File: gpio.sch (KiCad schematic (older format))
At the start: 7 parts, among them J1 DF40C-100DP-0.4V(51), J2 DF40C-100DP-0.4V(51), U1 LFE5U-85F-6BG381C

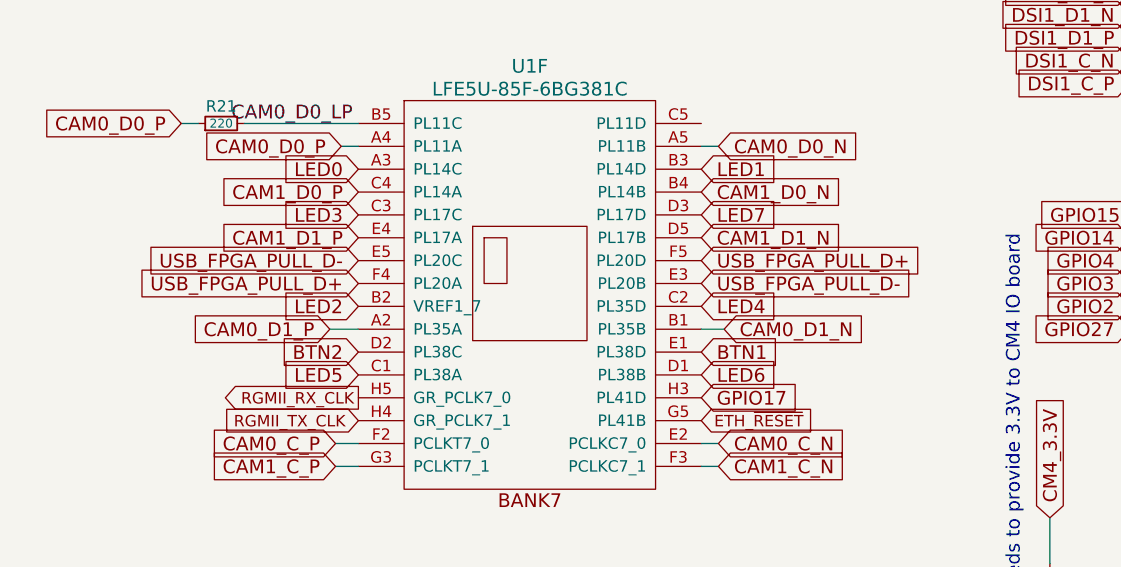
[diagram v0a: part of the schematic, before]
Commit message: Changing and routing USB pins fix #25
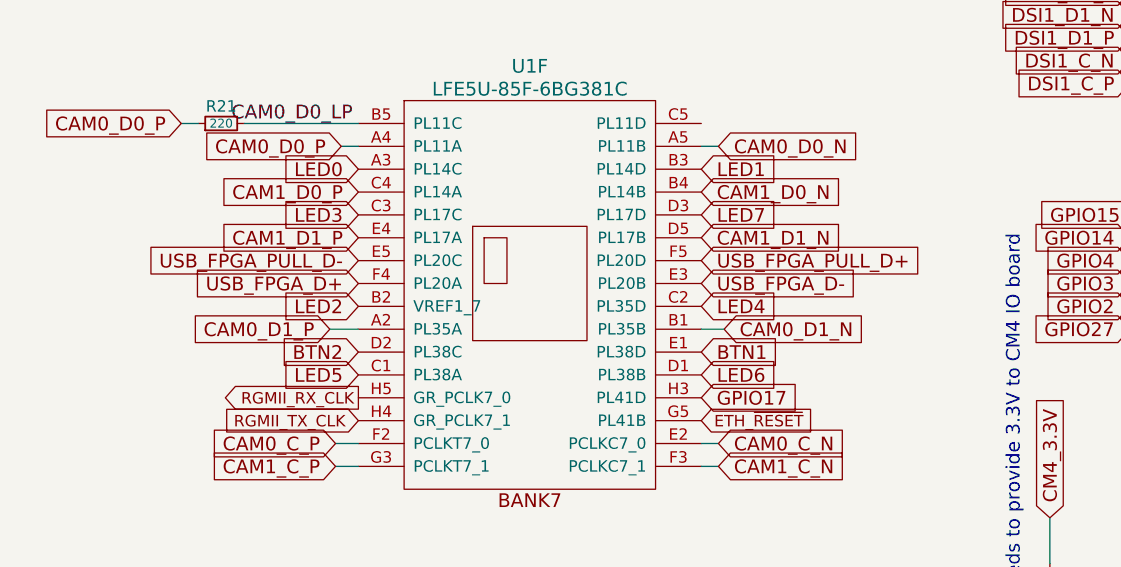
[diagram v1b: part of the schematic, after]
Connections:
- net USB_FPGA_D+: now also U1.F4 (PL20A)
- net USB_FPGA_D-: now also U1.E3 (PL20B)
- net USB_FPGA_PULL_D+: no longer U1.F4 (PL20A)
- net USB_FPGA_PULL_D-: no longer U1.E3 (PL20B)
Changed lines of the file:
@@
 LED1
 Text GLabel 1925 3950 0    60   Input ~ 0
-USB_FPGA_PULL_D+
+USB_FPGA_D+
 Text GLabel 3425 3950 2    60   Input ~ 0
-USB_FPGA_PULL_D-
+USB_FPGA_D-
 Text GLabel 1825 4750 0    60   Input ~ 0
 CAM1_C_P

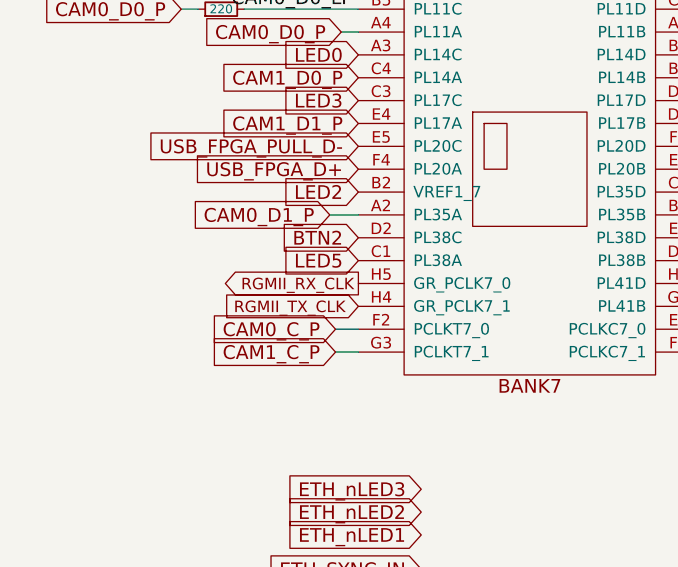
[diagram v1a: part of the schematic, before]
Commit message: Chaning RGMII_RX_CLK to H2, removing H5, adding pulldown to pin 33 fix #35
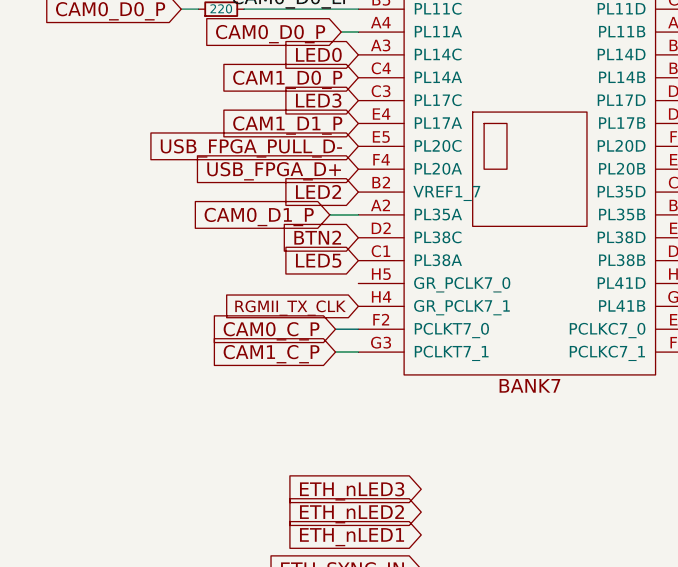
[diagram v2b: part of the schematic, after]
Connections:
- net RGMII_RX_CLK: no longer names the net of U1.H5 (GR_PCLK7_0)
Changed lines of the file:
@@
 Text GLabel 3425 4450 2    60   Input ~ 0
 GPIO17
-Text GLabel 1925 4450 0    50   Output ~ 0
-RGMII_RX_CLK
 Text GLabel 1925 4550 0    50   Input ~ 0
 RGMII_TX_CLK

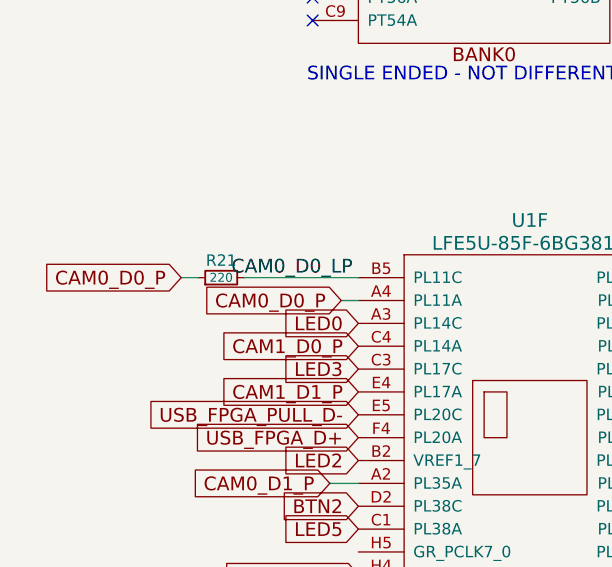
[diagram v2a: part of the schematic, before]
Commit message: Lowering number of unique parts fix #37
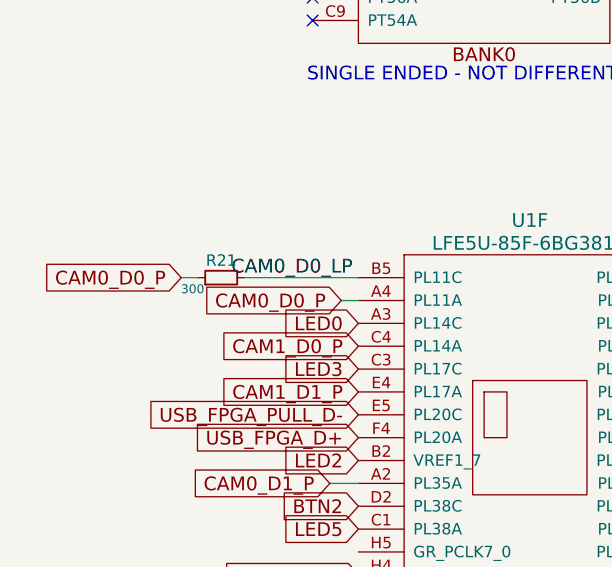
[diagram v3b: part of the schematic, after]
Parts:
- R21: value 220 -> 300
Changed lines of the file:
@@
 AR Path="/56AC389C/625E5FDB" Ref="R21"  Part="1"
 F 0 "R21" V 1400 3250 50  0000 C CNN
-F 1 "220" V 1325 3250 39  0000 C CNN
+F 1 "300" V 1275 3375 39  0000 C CNN
 F 2 "Resistor_SMD:R_0402_1005Metric" H 1325 3250 50  0001 C CNN
 F 3 "~" H 1325 3250 50  0001 C CNN

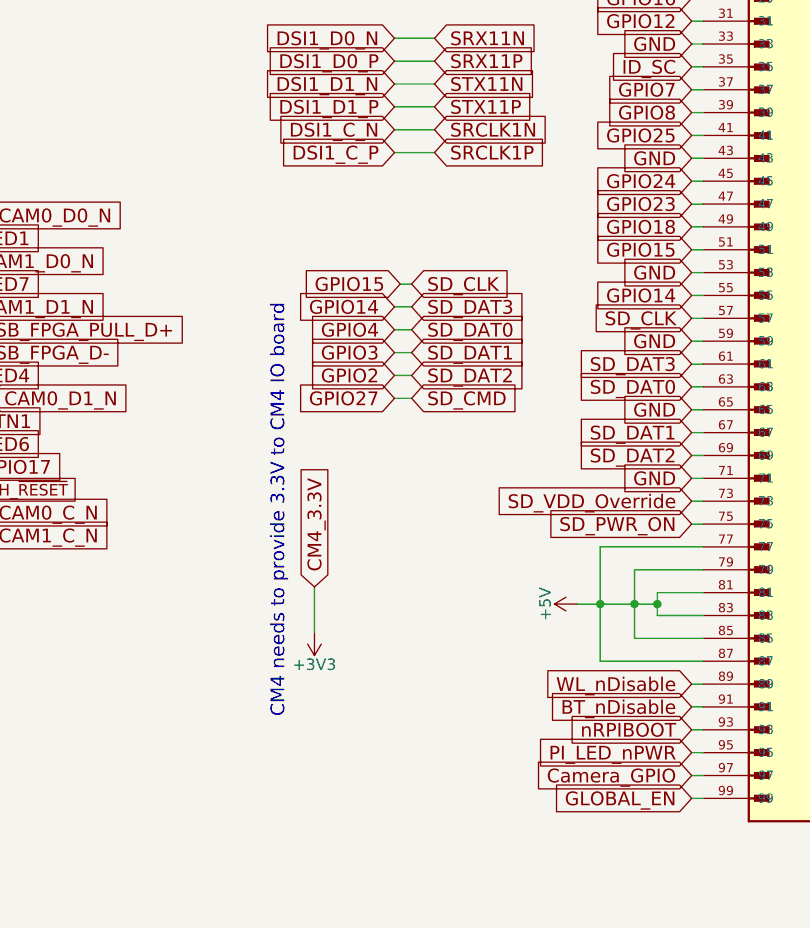
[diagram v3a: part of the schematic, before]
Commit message: Removing SD-CARD sharing feature to get more GPIO pins
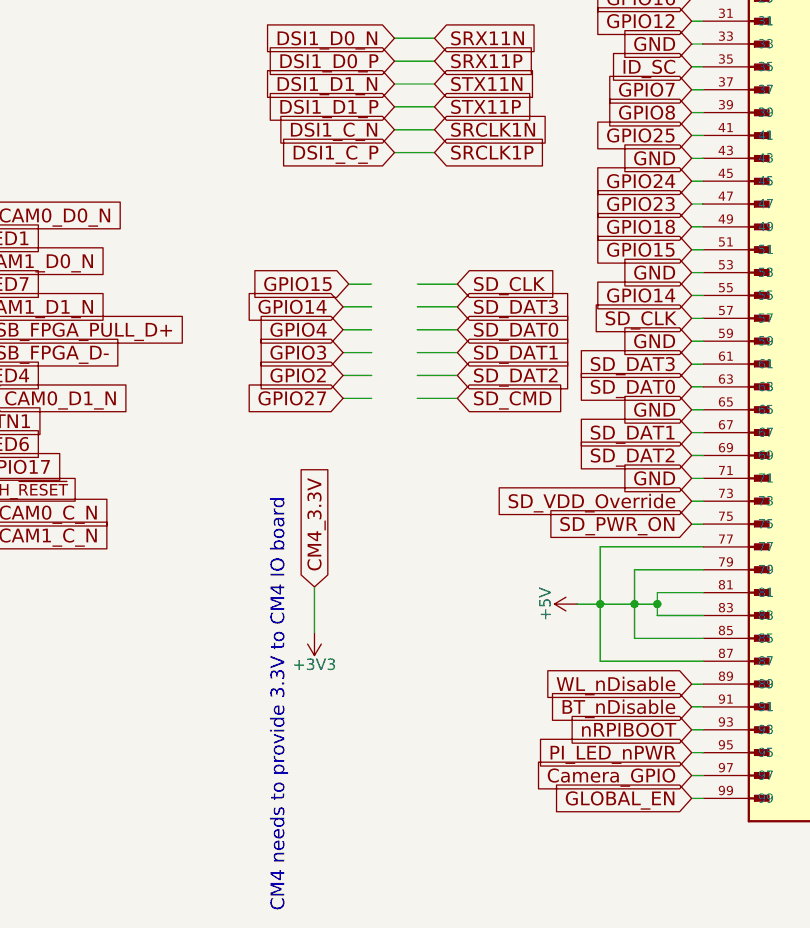
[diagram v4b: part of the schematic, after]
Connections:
- wire segments 232 -> 238
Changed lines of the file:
@@
 Wire Wire Line
 	4950 5175 4950 4975
-Text Notes 4825 5550 1    60   ~ 0
+Text Notes 4825 6400 1    60   ~ 0
 CM4 needs to provide 3.3V to CM4 IO board
 Text GLabel 5475 2675 2    60   Input ~ 0
@@
 Wire Wire Line
 	5475 3075 5300 3075
-Text GLabel 5325 3650 0    60   Input ~ 0
+Text GLabel 5100 3650 0    60   Input ~ 0
 GPIO15
-Text GLabel 5375 3650 2    60   Input ~ 0
+Text GLabel 5575 3650 2    60   Input ~ 0
 SD_CLK
-Wire Wire Line
-	5325 3650 5375 3650
-Text GLabel 5300 3750 0    60   Input ~ 0
+Text GLabel 5075 3750 0    60   Input ~ 0
 GPIO14
-Text GLabel 5375 3750 2    60   Input ~ 0
+Text GLabel 5575 3750 2    60   Input ~ 0
 SD_DAT3
-Wire Wire Line
-	5300 3750 5375 3750
-Text GLabel 5375 3850 2    60   Input ~ 0
+Text GLabel 5575 3850 2    60   Input ~ 0
 SD_DAT0
 Text GLabel 6600 4300 0    60   Input ~ 0
 SD_DAT1
-Text GLabel 5375 3950 2    60   Input ~ 0
+Text GLabel 5575 3950 2    60   Input ~ 0
 SD_DAT1
-Text GLabel 5375 4050 2    60   Input ~ 0
+Text GLabel 5575 4050 2    60   Input ~ 0
 SD_DAT2
-Text GLabel 5375 4150 2    60   Input ~ 0
+Text GLabel 5575 4150 2    60   Input ~ 0
 SD_CMD
-Text GLabel 5300 3850 0    60   Input ~ 0
+Text GLabel 5075 3850 0    60   Input ~ 0
 GPIO4
-Text GLabel 5300 3950 0    60   Input ~ 0
+Text GLabel 5075 3950 0    60   Input ~ 0
 GPIO3
-Text GLabel 5300 4050 0    60   Input ~ 0
+Text GLabel 5075 4050 0    60   Input ~ 0
 GPIO2
-Wire Wire Line
-	5300 3850 5375 3850
-Wire Wire Line
-	5375 3950 5300 3950
-Wire Wire Line
-	5300 4050 5375 4050
-Text GLabel 5300 4150 0    60   Input ~ 0
+Text GLabel 5075 4150 0    60   Input ~ 0
 GPIO27
-Wire Wire Line
-	5300 4150 5375 4150
 Text GLabel 2200 5350 0    60   Input ~ 0
 ETH_nLED3
@@
 Wire Wire Line
 	3225 1525 3500 1525
+Wire Wire Line
+	5400 3950 5575 3950
+Wire Wire Line
+	5400 4050 5575 4050
+Wire Wire Line
+	5400 4150 5575 4150
+Wire Wire Line
+	5075 3950 5200 3950
+Wire Wire Line
+	5075 4050 5200 4050
+Wire Wire Line
+	5075 4150 5200 4150
+Wire Wire Line
+	5075 3850 5200 3850
+Wire Wire Line
+	5400 3850 5575 3850
+Wire Wire Line
+	5075 3750 5200 3750
+Wire Wire Line
+	5400 3750 5575 3750
+Wire Wire Line
+	5100 3650 5200 3650
+Wire Wire Line
+	5400 3650 5575 3650
 $EndSCHEMATC

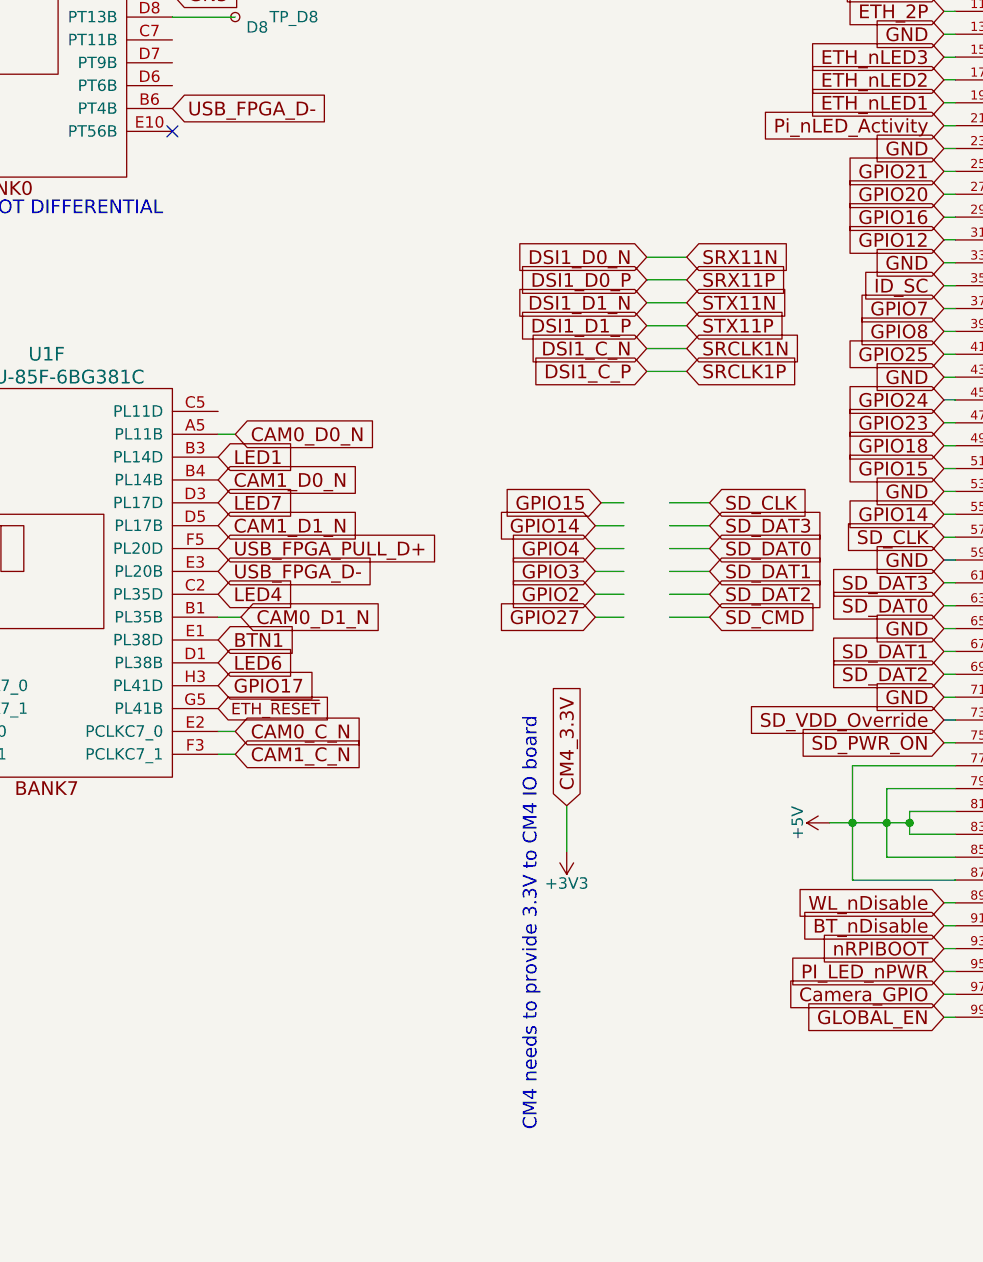
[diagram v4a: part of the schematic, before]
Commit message: Connecting DSI1 to DSI0
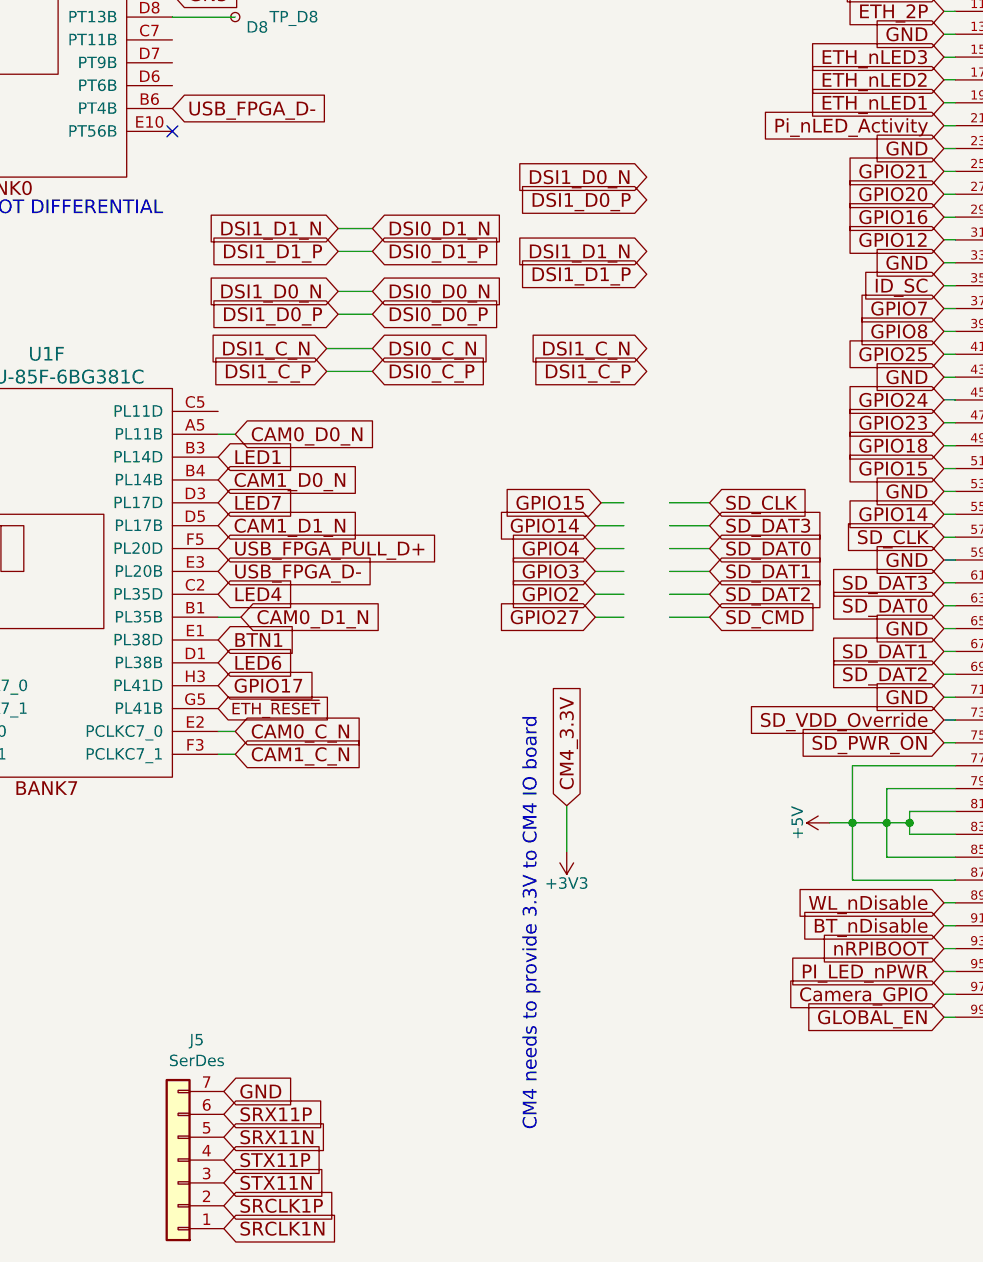
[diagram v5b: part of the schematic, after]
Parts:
- added J5: SerDes, Connector_PinHeader_1.00mm:PinHeader_1x07_P1.00mm_Vertical, symbol Connector_Generic:Conn_01x07
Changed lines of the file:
@@
 Text GLabel 5300 2975 0    60   Input ~ 0
 DSI1_C_N
-Text GLabel 5300 2875 0    60   Input ~ 0
+Text GLabel 5300 2650 0    60   Input ~ 0
 DSI1_D1_P
-Text GLabel 5300 2775 0    60   Input ~ 0
+Text GLabel 5300 2550 0    60   Input ~ 0
 DSI1_D1_N
-Text GLabel 5300 2675 0    60   Input ~ 0
+Text GLabel 5300 2325 0    60   Input ~ 0
 DSI1_D0_P
-Text GLabel 5300 2575 0    60   Input ~ 0
+Text GLabel 5300 2225 0    60   Input ~ 0
 DSI1_D0_N
 Text GLabel 3425 3850 2    60   Input ~ 0
@@
 Text Notes 4825 6400 1    60   ~ 0
 CM4 needs to provide 3.3V to CM4 IO board
-Text GLabel 5475 2675 2    60   Input ~ 0
+Text GLabel 3450 6325 2    60   Input ~ 0
 SRX11P
-Text GLabel 5475 2575 2    60   Input ~ 0
+Text GLabel 3450 6425 2    60   Input ~ 0
 SRX11N
-Text GLabel 5475 2875 2    60   Input ~ 0
+Text GLabel 3450 6525 2    60   Input ~ 0
 STX11P
-Text GLabel 5475 2775 2    60   Input ~ 0
+Text GLabel 3450 6625 2    60   Input ~ 0
 STX11N
-Text GLabel 5475 3075 2    60   Input ~ 0
+Text GLabel 3450 6725 2    60   Input ~ 0
 SRCLK1P
-Text GLabel 5475 2975 2    60   Input ~ 0
+Text GLabel 3450 6825 2    60   Input ~ 0
 SRCLK1N
-Wire Wire Line
-	5300 2575 5475 2575
-Wire Wire Line
-	5475 2675 5300 2675
-Wire Wire Line
-	5300 2775 5475 2775
-Wire Wire Line
-	5475 2875 5300 2875
-Wire Wire Line
-	5300 2975 5475 2975
-Wire Wire Line
-	5475 3075 5300 3075
 Text GLabel 5100 3650 0    60   Input ~ 0
 GPIO15
@@
 Wire Wire Line
 	5400 3650 5575 3650
+Text GLabel 3900 3075 0    60   Input ~ 0
+DSI1_C_P
+Text GLabel 3900 2975 0    60   Input ~ 0
+DSI1_C_N
+Text GLabel 4100 3075 2    60   Input ~ 0
+DSI0_C_P
+Text GLabel 4100 2975 2    60   Input ~ 0
+DSI0_C_N
+Wire Wire Line
+	3900 2975 4100 2975
+Wire Wire Line
+	4100 3075 3900 3075
+Text GLabel 3950 2825 0    60   Input ~ 0
+DSI1_D0_P
+Text GLabel 3950 2725 0    60   Input ~ 0
+DSI1_D0_N
+Text GLabel 3950 2550 0    60   Input ~ 0
+DSI1_D1_P
+Text GLabel 3950 2450 0    60   Input ~ 0
+DSI1_D1_N
+Text GLabel 4100 2825 2    60   Input ~ 0
+DSI0_D0_P
+Text GLabel 4100 2725 2    60   Input ~ 0
+DSI0_D0_N
+Text GLabel 4100 2550 2    60   Input ~ 0
+DSI0_D1_P
+Text GLabel 4100 2450 2    60   Input ~ 0
+DSI0_D1_N
+Wire Wire Line
+	3950 2450 4100 2450
+Wire Wire Line
+	4100 2550 3950 2550
+Wire Wire Line
+	3950 2725 4100 2725
+Wire Wire Line
+	4100 2825 3950 2825
+$Comp
+L Connector_Generic:Conn_01x07 J5
+U 1 1 63CD0255
+P 3250 6525
+F 0 "J5" H 3168 6000 50  0000 C CNN
+F 1 "SerDes" H 3168 6091 50  0000 C CNN
+F 2 "Connector_PinHeader_1.00mm:PinHeader_1x07_P1.00mm_Vertical" H 3250 6525 50  0001 C CNN
+F 3 "~" H 3250 6525 50  0001 C CNN
+	1    3250 6525
+	-1   0    0    1
+$EndComp
+Text GLabel 3450 6225 2    60   Input ~ 0
+GND
 $EndSCHEMATC
